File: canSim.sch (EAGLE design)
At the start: 16 parts

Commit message: New revision with new OBD-2.  Auto PCB routing to still change.
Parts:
- U$9: value OBD_2FEMALE -> OBD_2FEMALEOBD2_FEMALE_PTH; device OBD2_Female_PTH:OBD_2FEMALE -> OBD2_Female_PTH:OBD_2FEMALEOBD2_FEMALE_PTH
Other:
- moved on the sheet: H1, H2, H3, H4, H5, U$1

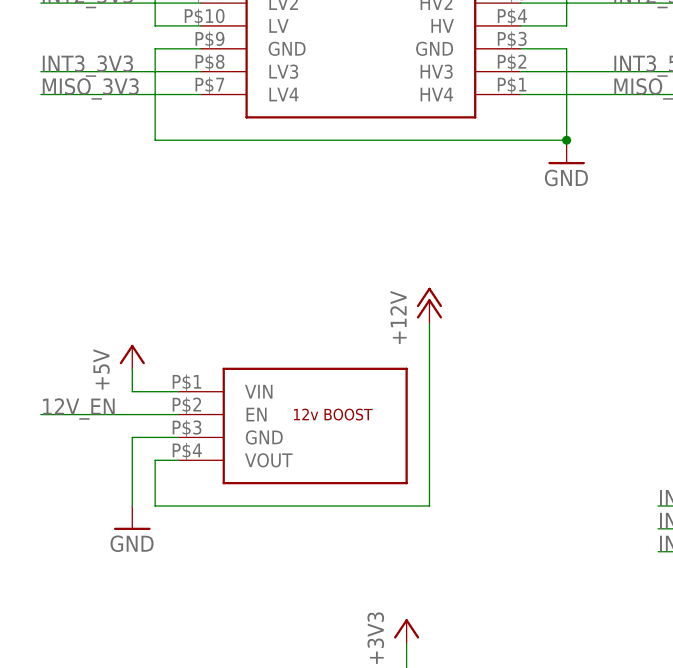
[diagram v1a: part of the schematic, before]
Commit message: Release candidate
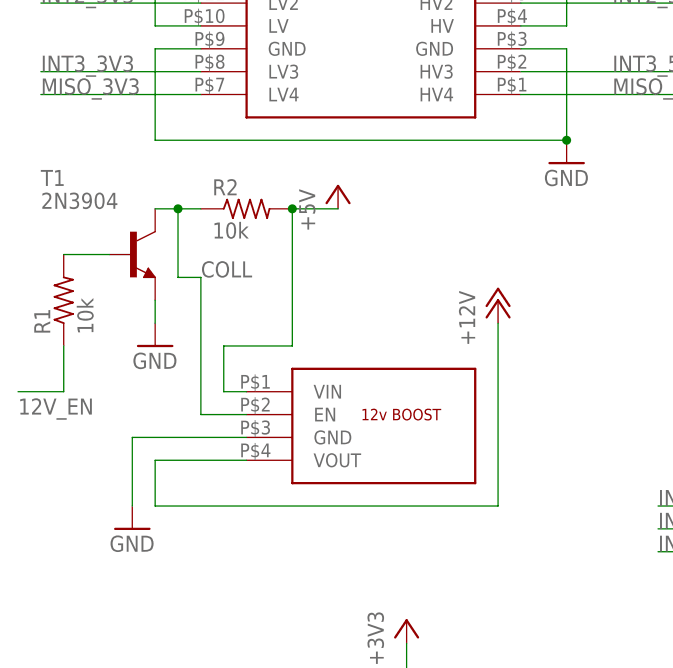
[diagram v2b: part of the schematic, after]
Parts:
- added R1, R2: 10k, resistor:R-US_0207/2V
- added T1: 2N3904, transistor:2N3904
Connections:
- new net COLL: R2.1, T1.C, U$6.EN
- new net N$2: R1.2, T1.B
- net +5V: now also R2.2
- net 12V_EN: now also R1.1; no longer U$6.EN
- net GND: now also T1.E
